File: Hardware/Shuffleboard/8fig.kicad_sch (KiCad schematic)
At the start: 22 parts

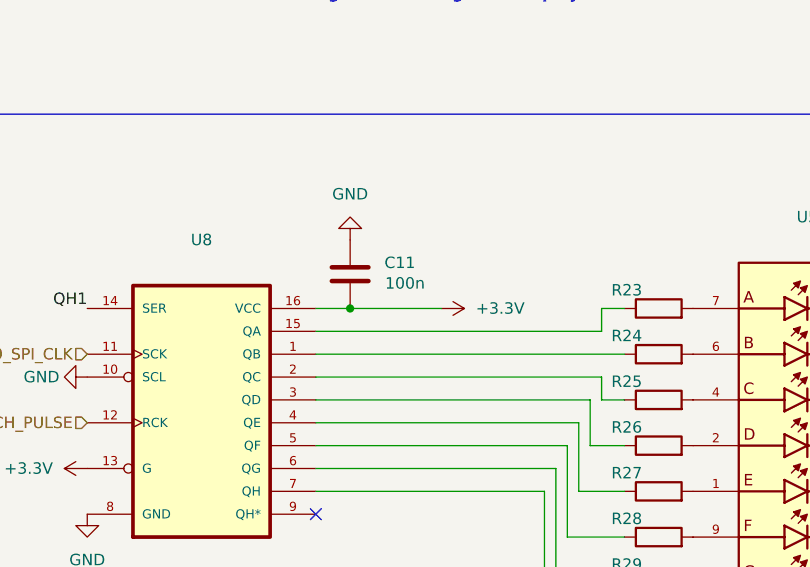
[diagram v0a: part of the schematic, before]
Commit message: updated to end
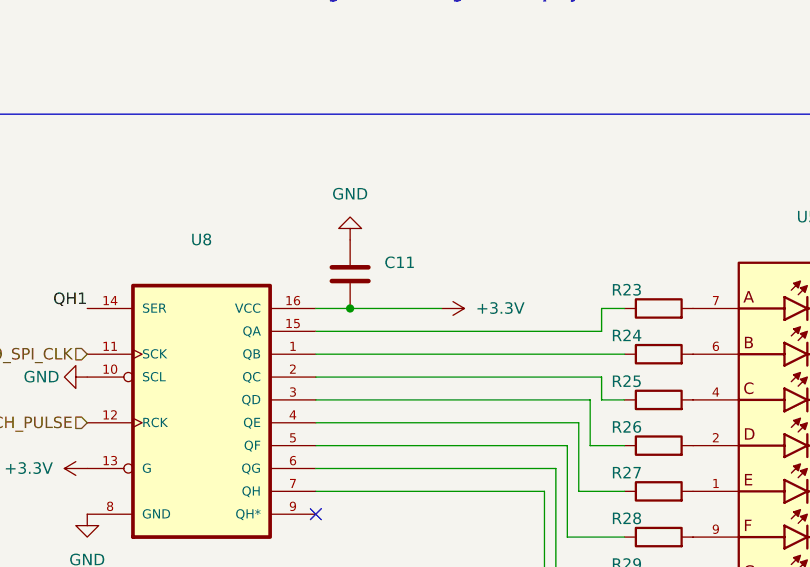
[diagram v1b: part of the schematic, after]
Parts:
- C10, C11: value 100n -> (none)
- R15, R16, R17, R18, R19, R20, R21, R22, R23, R24, R25, R26, R27, R28, R29, R30: value 100 -> (none)
